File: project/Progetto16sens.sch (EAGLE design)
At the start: 148 parts, among them IC1 LMZ14202TZE-ADJ_NOPB, J2 455-1750-1-ND, M1 43650-0201, M2 43650-0201, M3 43650-0201, M4 43650-0201, M5 ARDUINO-PRO-MINI, SW1 TL32PO, SW2 TL32PO, SW3 TL32PO

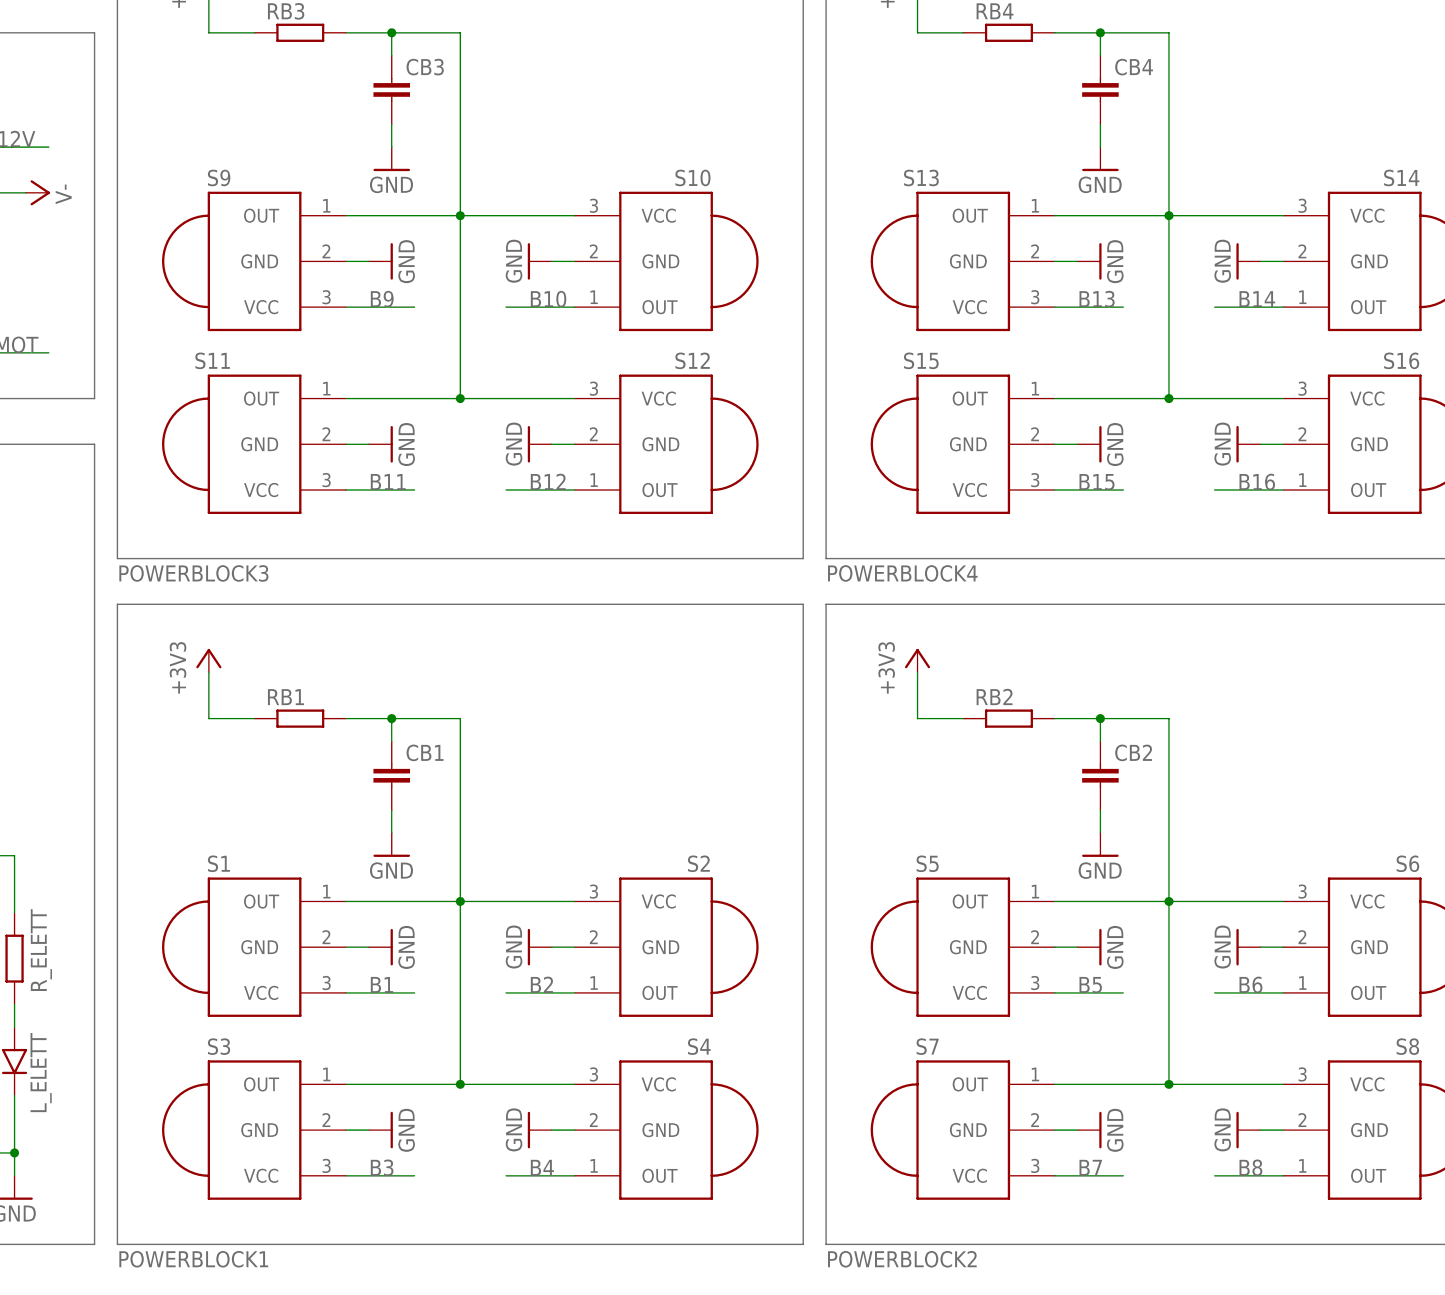
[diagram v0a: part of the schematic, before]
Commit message: turned in elaborato
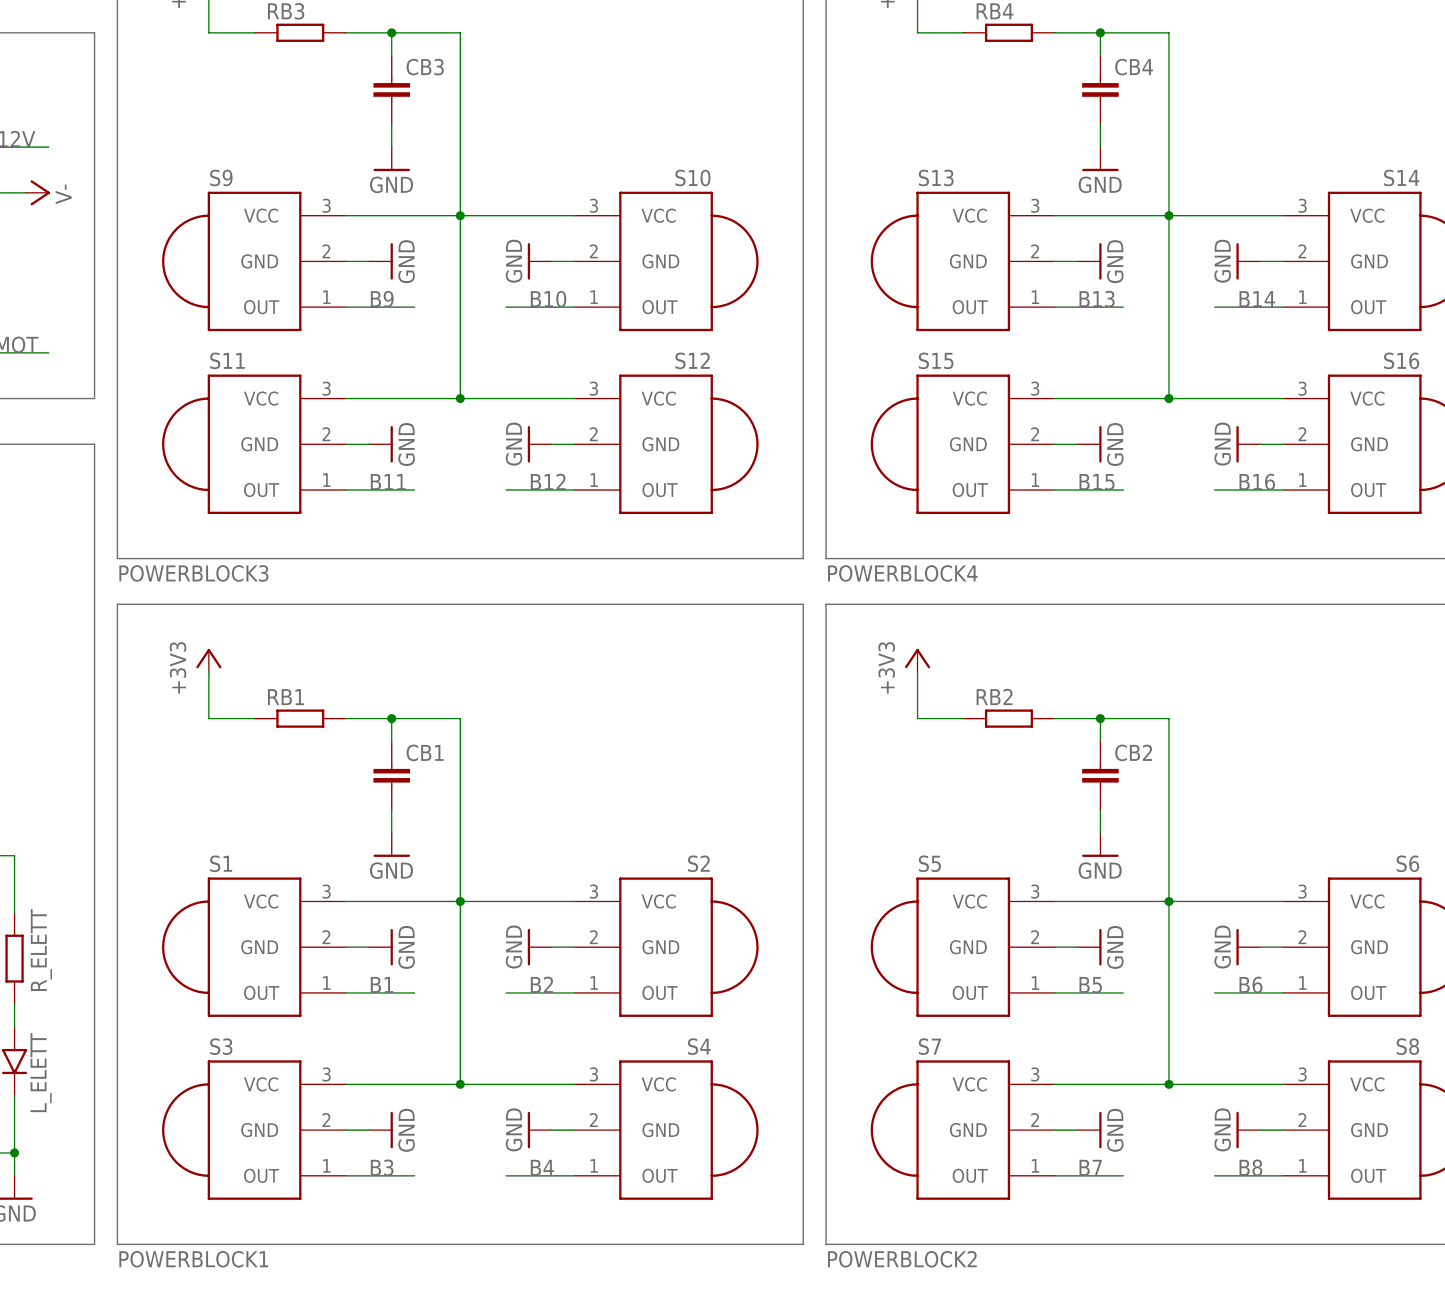
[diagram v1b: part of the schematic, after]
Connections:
- removed net N$1: CB2.1, RB2.2, S5.OUT, S6.VCC, S7.OUT, S8.VCC
- removed net N$2: CB1.1, RB1.2, S1.OUT, S2.VCC, S3.OUT, S4.VCC
- removed net N$3: CB3.1, RB3.2, S10.VCC, S11.OUT, S12.VCC, S9.OUT
- removed net N$4: CB4.1, RB4.2, S13.OUT, S14.VCC, S15.OUT, S16.VCC
- removed net N$69: SV1.12, SV3.10, SV6.11, U$1.GND, U$1.GND_1, U$1.GND_2
- new net PWR_B1: CB1.1, RB1.2, S1.VCC, S2.VCC, S3.VCC, S4.VCC
- new net PWR_B2: CB2.1, RB2.2, S5.VCC, S6.VCC, S7.VCC, S8.VCC
- new net PWR_B3: CB3.1, RB3.2, S10.VCC, S11.VCC, S12.VCC, S9.VCC
- new net PWR_B4: CB4.1, RB4.2, S13.VCC, S14.VCC, S15.VCC, S16.VCC
- net B1: now also S1.OUT; no longer S1.VCC
- net B11: now also S11.OUT; no longer S11.VCC
- net B13: now also S13.OUT; no longer S13.VCC
- net B15: now also S15.OUT; no longer S15.VCC
- net B3: now also S3.OUT; no longer S3.VCC
- net B5: now also S5.OUT; no longer S5.VCC
- net B7: now also S7.OUT; no longer S7.VCC
- net B9: now also S9.OUT; no longer S9.VCC
- net GND: now also SV1.12, SV3.10, SV6.11, U$1.GND, U$1.GND_1, U$1.GND_2
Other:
- moved on the sheet: S1, S11, S13, S15, S3, S5, S7, S9
